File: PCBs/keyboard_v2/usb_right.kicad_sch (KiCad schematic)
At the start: 22 parts, among them J601 USB4510-03-1-A, J602 USB4510-03-1-A, J603 GSB12J21C1EU, U601 USBLC6-4SC6, U602 USBLC6-4SC6, U603 USBLC6-4SC6, U604 STM32G0B1KBUx, U605 USB2533-1080AEN, Y601 CX2016SA24000D0HLLG3

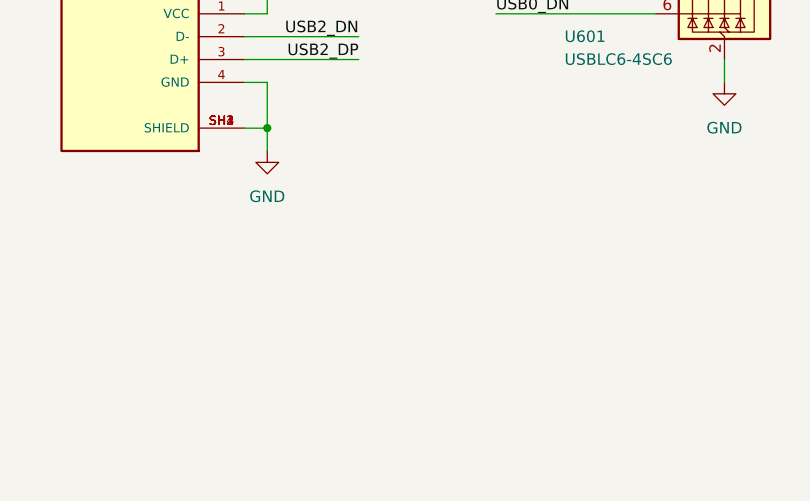
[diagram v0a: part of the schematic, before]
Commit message: Layout progress
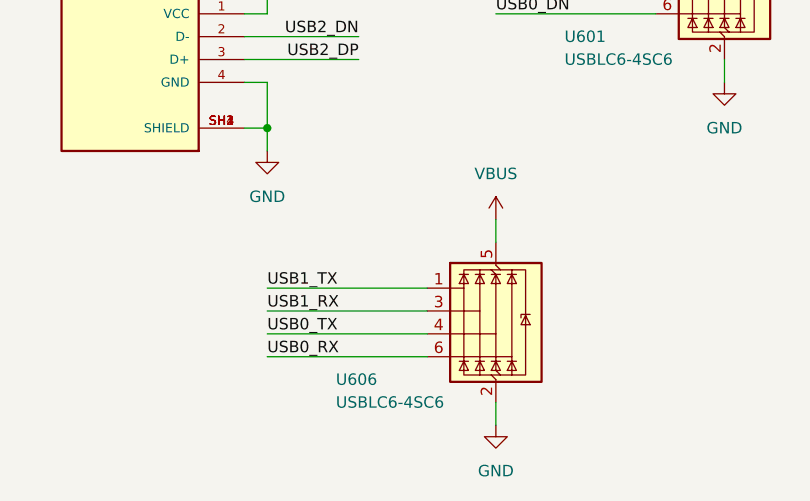
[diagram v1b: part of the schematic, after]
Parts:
- added U606: USBLC6-4SC6, Package_TO_SOT_SMD:SOT-23-6, symbol Power_Protection:USBLC6-4SC6
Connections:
- net GND: now also U606.2 (GND)
- net USB0_RX: now also U606.6 (I/O4)
- net USB0_TX: now also U606.4 (I/O3)
- net USB1_RX: now also U606.3 (I/O2)
- net USB1_TX: now also U606.1 (I/O1)
- net VBUS: now also U606.5 (VBUS)
